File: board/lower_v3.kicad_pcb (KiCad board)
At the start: 2 copper layers, 43.2 x 64.8 mm, 79 parts, among them J1 POWER, J10 PIN_RING_MOTOR, J11 PIN_PINKY_MOTOR, J12 PIN_PINKY_SPLAY, J13 PIN_RING_SPLAY, J14 PIN_MIDDLE_SPLAY, J15 PIN_INDEX_SPLAY, J16 PIN_THUMB_SPLAY, J17 PIN_A_BTN, J18 PIN_B_BTN, J19 JOYSTICK, J2 PIN_PINKY, J3 PIN_RING, J4 PIN_MIDDLE, J5 PIN_INDEX, J6 PIN_THUMB, J7 PIN_THUMB_MOTOR, J8 PIN_INDEX_MOTOR, J9 PIN_MIDDLE_MOTOR, U1 ESP32-DEVKIT-V1

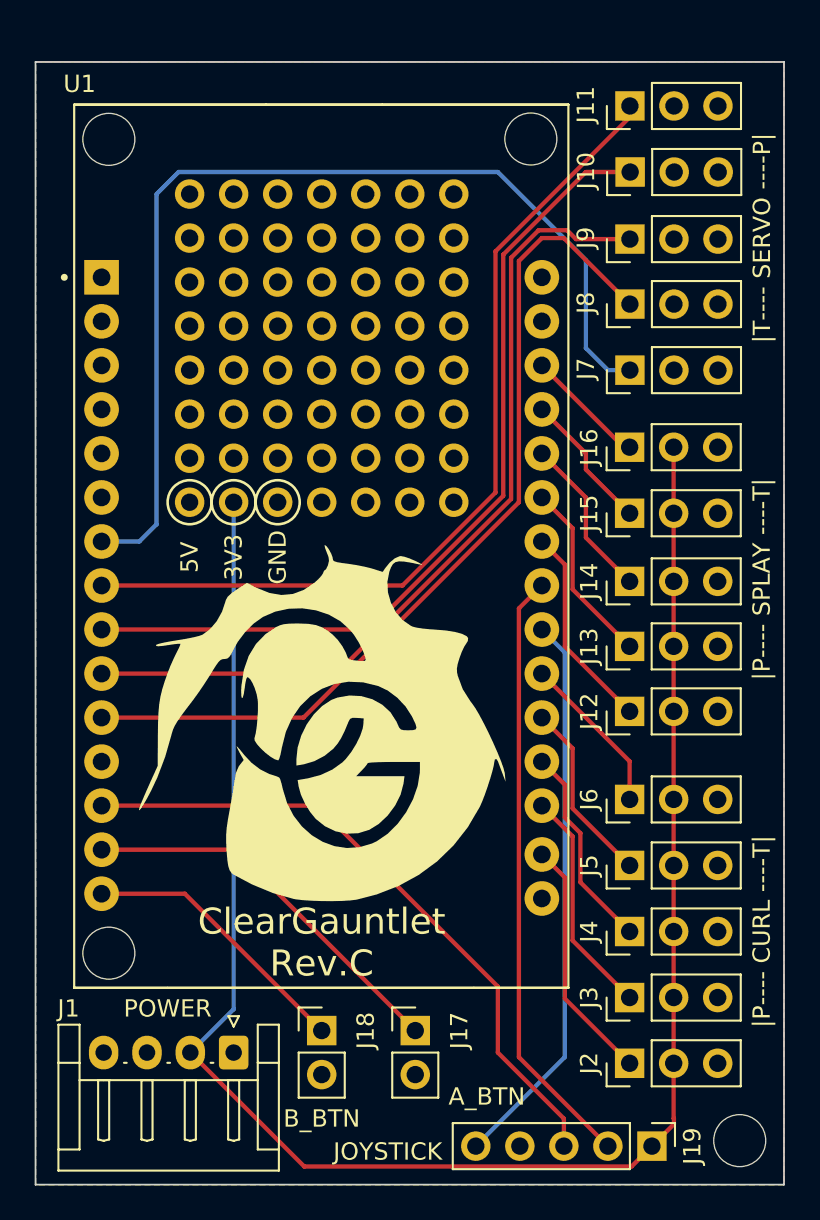
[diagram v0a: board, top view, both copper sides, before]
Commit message: RevC RC 1
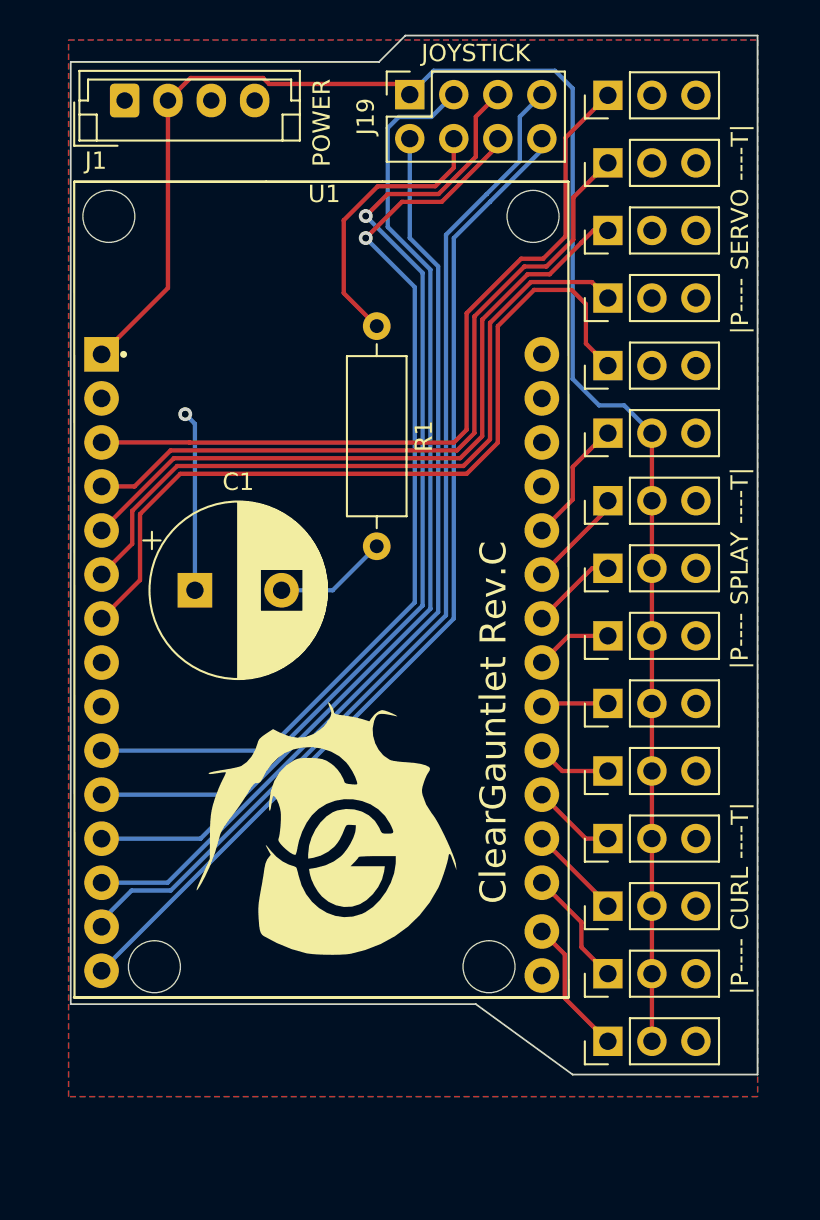
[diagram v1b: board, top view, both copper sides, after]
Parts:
- removed 83 (x24), 84 (x32), ? (x2): , 
- removed J17: PIN_A_BTN, Connector_PinHeader_2.54mm:PinHeader_1x02_P2.54mm_Vertical
- removed J18: PIN_B_BTN, Connector_PinHeader_2.54mm:PinHeader_1x02_P2.54mm_Vertical
- removed logo: LOGO, CG:logo-big
- added C1: C_Polarized, Capacitor_THT:CP_Radial_D10.0mm_P5.00mm, F.Cu at (122.2, 96.5)
- added G***: LOGO, cg_logo_small:cg_logo_med, F.Cu at (129.8, 110.2)
- added R1: R_US, Resistor_THT:R_Axial_DIN0309_L9.0mm_D3.2mm_P12.70mm_Horizontal, F.Cu at (132.7, 81.3)
- J1: footprint Connector_JST:JST_EH_S4B-EH_1x04_P2.50mm_Horizontal -> Connector_JST:JST_EH_B4B-EH-A_1x04_P2.50mm_Vertical
- J19: value JOYSTICK -> Conn_01x08_Male; footprint Connector_PinHeader_2.54mm:PinHeader_1x05_P2.54mm_Vertical -> Connector_PinSocket_2.54mm:PinSocket_2x04_P2.54mm_Vertical
- moved J19 62.3 mm to (134.6, 67.9), turned to 90 degrees
- moved J1 55.3 mm to (118.2, 68.3), turned to 0 degrees
- moved J7 15.9 mm to (146.1, 68.0)
- moved J11 15.0 mm to (146.1, 83.6)
- moved J8 8.25 mm to (146.1, 71.9)
- moved J10 7.38 mm to (146.1, 79.7)
- moved U1 4.44 mm to (129.5, 98.4)
- moved J6 2.06 mm to (146.1, 106.9)
- moved J5 2.00 mm to (146.1, 110.8)
- moved J4 1.93 mm to (146.1, 114.7)
- moved J3 1.86 mm to (146.1, 118.6)
- moved J2 1.79 mm to (146.1, 122.5)
- moved J16 1.49 mm to (146.1, 87.5)
- moved J14 1.46 mm to (146.1, 95.3)
- moved J15 1.45 mm to (146.1, 91.4)
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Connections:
- J10 pad 1: Net-(J10-Pad1) -> Net-(U1-Pad25)
- J12 pad 1: Net-(U1-Pad15) -> Net-(J12-Pad1)
- J13 pad 1: Net-(U1-Pad16) -> Net-(J13-Pad1)
- J14 pad 1: Net-(U1-Pad17) -> Net-(J14-Pad1)
- J16 pad 1: /Net-(U1-Pad20) -> Net-(J16-Pad1)
- J19 pad 3: Net-(U1-Pad41) -> Net-(J19-Pad3)
- J7 pad 1: Net-(J7-Pad1) -> Net-(U1-Pad21)
- J8 pad 1: Net-(J8-Pad1) -> Net-(U1-Pad22)
- J9 pad 1: Net-(J9-Pad1) -> Net-(U1-Pad24)
- U1 pad 102: GND -> unconnected-(U1-Pad102)
- U1 pad 103: /5V -> unconnected-(U1-Pad103)
- U1 pad 104: unconnected-(U1-Pad104) -> /3V3
- U1 pad 13: Net-(J19-Pad5) -> Net-(J12-Pad1)
- U1 pad 14: Net-(J19-Pad2) -> Net-(J13-Pad1)
- U1 pad 15: Net-(U1-Pad15) -> Net-(J14-Pad1)
- U1 pad 16: Net-(U1-Pad16) -> Net-(J15-Pad1)
- U1 pad 17: Net-(U1-Pad17) -> Net-(J16-Pad1)
- U1 pad 18: Net-(J15-Pad1) -> unconnected-(U1-Pad18)
- U1 pad 21: unconnected-(U1-Pad21) -> Net-(U1-Pad21)
- U1 pad 22: unconnected-(U1-Pad22) -> Net-(U1-Pad22)
- U1 pad 24: unconnected-(U1-Pad24) -> Net-(U1-Pad24)
- U1 pad 25: unconnected-(U1-Pad25) -> Net-(U1-Pad25)
- U1 pad 27: Net-(J7-Pad1) -> Net-(J11-Pad1)
- U1 pad 34: Net-(J11-Pad1) -> unconnected-(U1-Pad34)
- U1 pad 35: Net-(J10-Pad1) -> unconnected-(U1-Pad35)
- U1 pad 36: Net-(U1-Pad36) -> Net-(J19-Pad8)
- U1 pad 38: Net-(J9-Pad1) -> Net-(J19-Pad6)
- U1 pad 39: Net-(U1-Pad39) -> Net-(J19-Pad7)
- U1 pad 40: unconnected-(U1-Pad40) -> Net-(J19-Pad3)
- U1 pad 41: Net-(U1-Pad41) -> Net-(J19-Pad2)
- U1 pad 42: Net-(J8-Pad1) -> Net-(J19-Pad5)
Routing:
- net Net-(J19-Pad7): track 0.00 -> 59.9 mm
- net Net-(J19-Pad8): track 0.00 -> 58.5 mm
- net Net-(J7-Pad1): track 58.2 -> 0.00 mm
- net Net-(J19-Pad3): track 0.00 -> 57.8 mm
- net Net-(J19-Pad6): track 0.00 -> 54.0 mm, vias 0 -> 1
- net Net-(J8-Pad1): track 51.7 -> 0.00 mm
- net Net-(J10-Pad1): track 49.6 -> 0.00 mm
- net Net-(J9-Pad1): track 49.4 -> 0.00 mm
- net Net-(U1-Pad21): track 0.00 -> 44.8 mm
- net Net-(U1-Pad22): track 0.00 -> 42.3 mm
- net Net-(U1-Pad25): track 0.00 -> 41.6 mm
- net Net-(U1-Pad24): track 0.00 -> 40.3 mm
- net Net-(U1-Pad41): track 38.0 -> 0.00 mm
- net Net-(J19-Pad5): track 32.5 -> 58.7 mm, vias 0 -> 1
- net Net-(U1-Pad39): track 22.4 -> 0.00 mm
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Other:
- board size 43.2 x 64.8 mm -> 39.6 x 59.9 mm
- board text added: "Bruh."
- board text added: "|P---- SERVO ----T|"
- board text removed: "A_BTN"
- board text removed: "B_BTN"
- board text removed: "|T---- SERVO ----P|"
